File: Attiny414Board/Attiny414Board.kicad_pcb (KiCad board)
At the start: 2 copper layers, 21 x 30.5 mm, 13 parts, among them J1 programming connector, J2 right connector, J4 Conn_01x04, U1 ATtiny414-SS

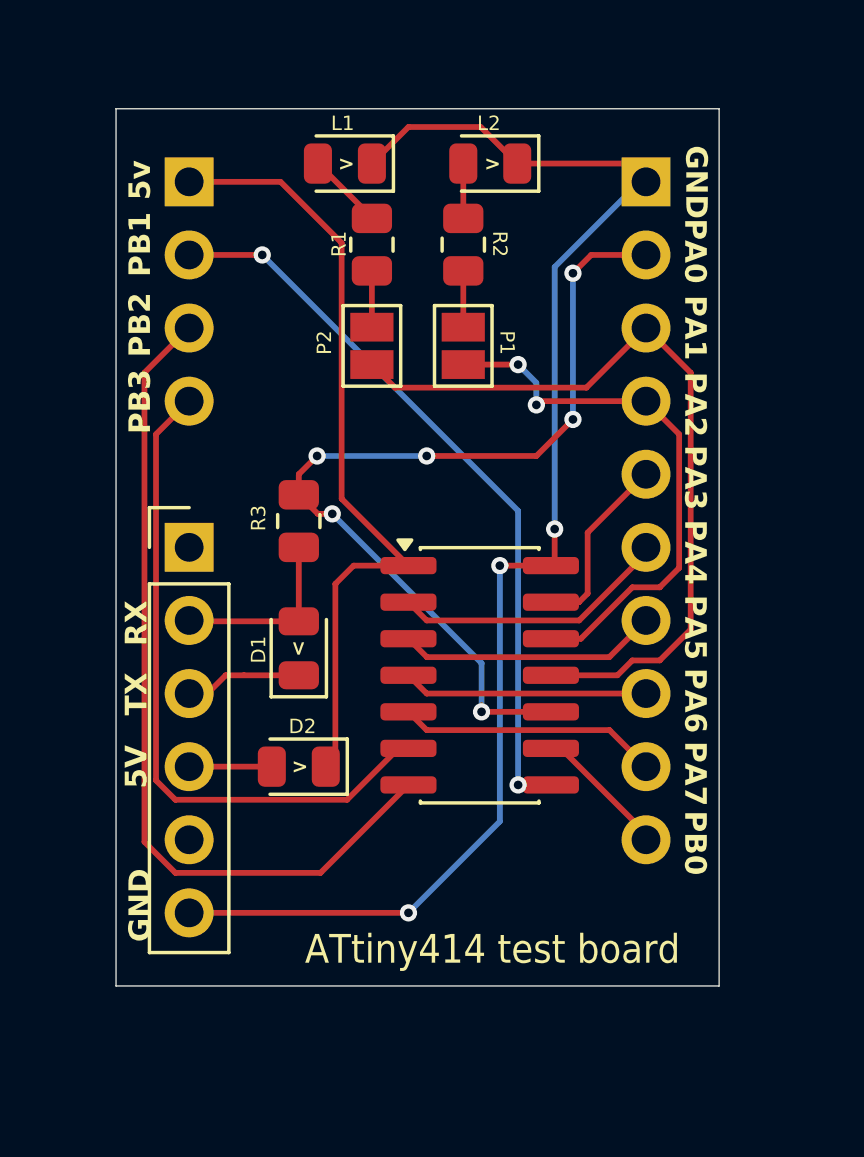
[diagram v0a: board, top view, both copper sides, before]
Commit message: Updated board
Updated the board from the feedback
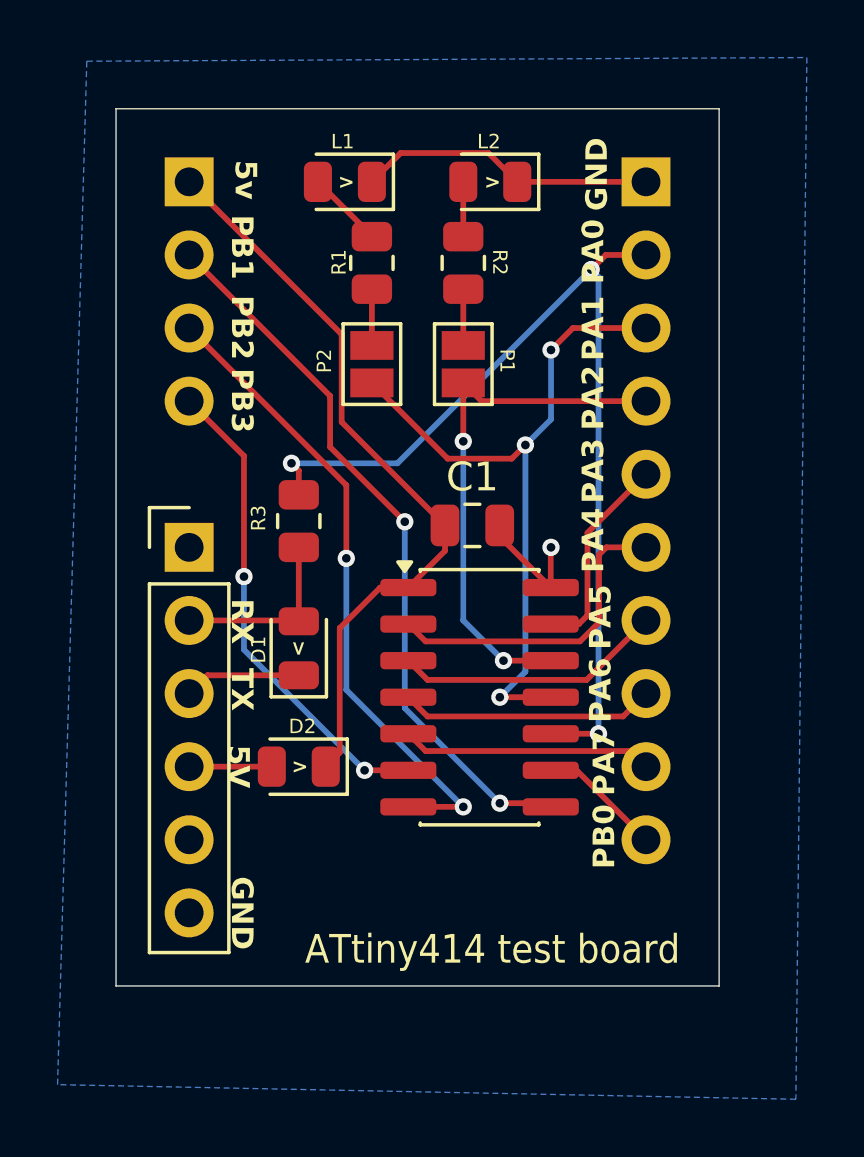
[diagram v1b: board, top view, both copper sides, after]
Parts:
- added C1: C, Capacitor_SMD:C_0805_2012Metric, F.Cu at (35.2, 39.2)
- moved U1 0.76 mm to (35.5, 45.2)
- moved JP1 0.63 mm to (31.8, 33.6)
- moved JP2 0.63 mm to (34.9, 33.6)
- moved L1 0.63 mm to (30.8, 27.3)
- moved L2 0.63 mm to (35.9, 27.3)
- moved R1 0.63 mm to (31.8, 30.1)
- moved R2 0.63 mm to (34.9, 30.1)
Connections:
- net 0 renamed gnd
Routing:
- net gnd: track 48.4 -> 14.6 mm, vias 3 -> 1
- net PB2: track 29.4 -> 22.5 mm, vias 0 -> 2
- net PB3: track 23.4 -> 16.9 mm, vias 0 -> 2
- net PA1: track 27.3 -> 24.8 mm, vias 0 -> 3
- net RESET*/PA0: track 32.0 -> 34.4 mm, vias 6 -> 3
- net PA4: track 9.70 -> 11.2 mm
- net +5V: track 27.6 -> 26.3 mm
- net PA3: track 6.39 -> 7.15 mm
- net PA2: track 19.2 -> 18.5 mm
- added copper zone on B.Cu, net gnd
